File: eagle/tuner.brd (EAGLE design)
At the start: 42.8 x 53.3 mm, 32 parts, among them IC1 MEGA8-AI, IC2 LM358D, IC3 7805TV, M1 MIC

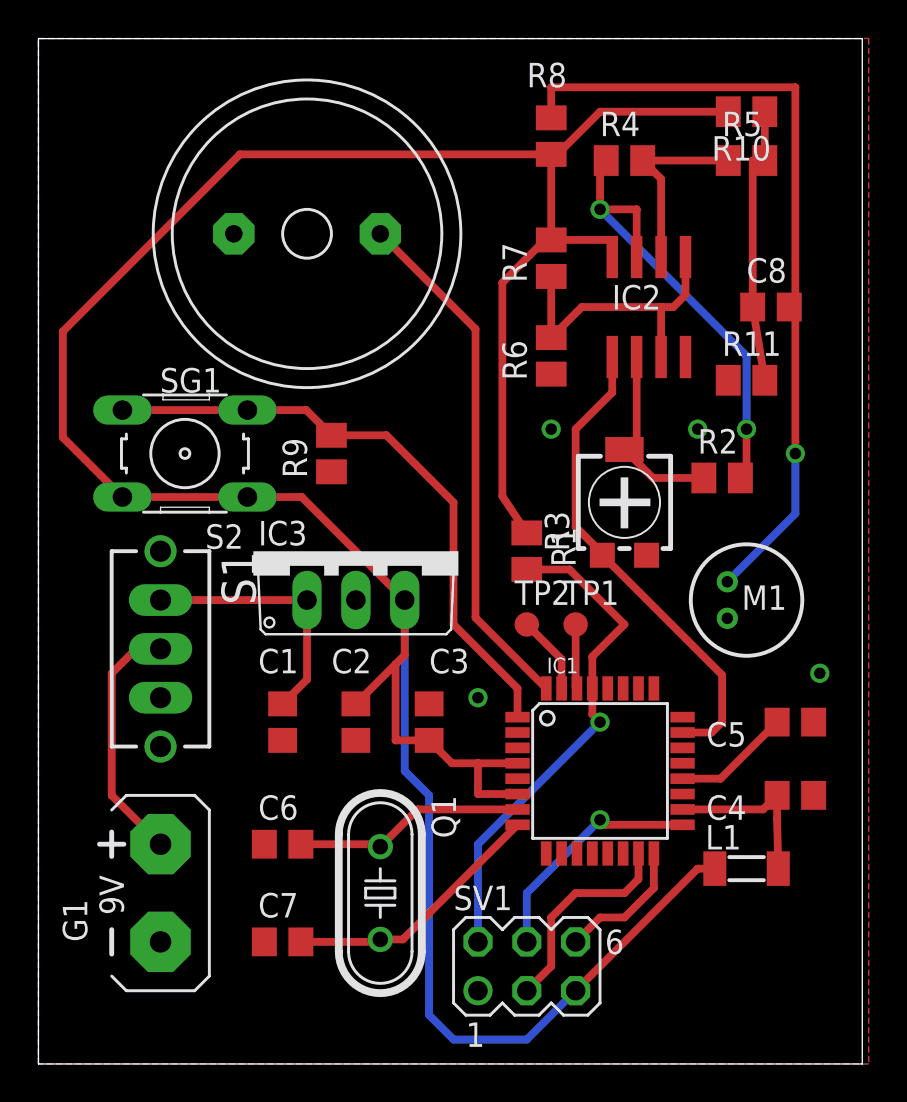
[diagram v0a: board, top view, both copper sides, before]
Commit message: updated PCB
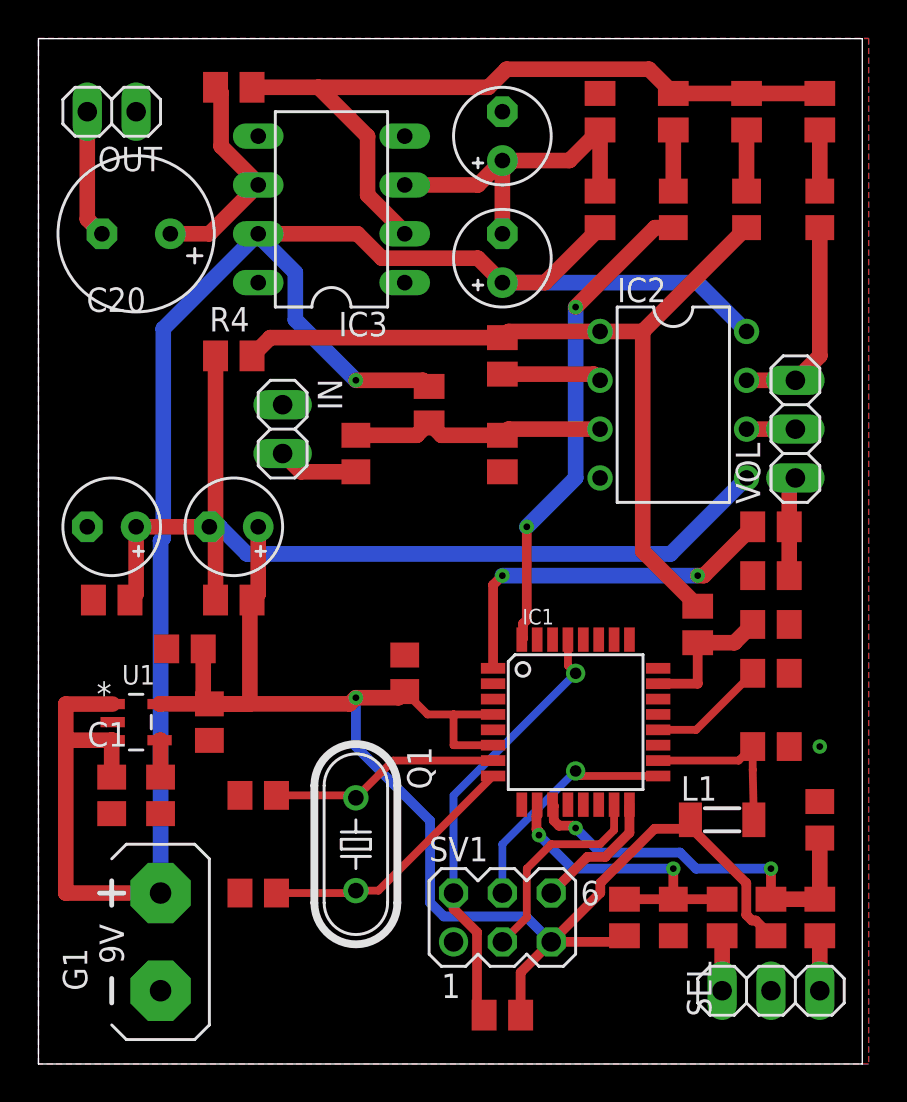
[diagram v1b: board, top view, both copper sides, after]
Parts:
- removed M1: MIC, microphon:WM-64PN
- removed S1: POWER, switch:TL3XYO
- removed S2: (no value), switch-omron:B3F-10XX
- removed SG1: BUZZER, buzzer:F/QMB
- removed TP1, TP2: PTR1B1,27, testpad:B1,27
- added C10, C14, C15, C22, C23: 0.1uF, eagle-ltspice:C0805
- added C11, C12, C13: 1uF, eagle-ltspice:C0805
- added C16, C17, C18, C19: 47uF, rcl:E2,5-5
- added C20: 470uF, rcl:E3,5-8
- added C9: 470pF, eagle-ltspice:C0805
- added IN, OUT: (no value), pinhead:1X02
- added R12, R13, R16, R17, R18, R19: 10k, resistor:M0805
- added R14, R15: 1k, resistor:M0805
- added SEL, VOL: (no value), pinhead:1X03
- added U1: LP2985AIM5-5.0, LP2985AIM5-5.0:SOT95P284X119-5N
- C2: value 0.1uF -> 2.2uF
- IC2: value LM358D -> LM358N; device linear:SO08 -> linear:DIL08
- IC3: value 7805TV -> AD811N; device linear:TO220V -> analog-devices:DIL08
- R10, R4: value 220k -> 10k
- R11: value 220k -> 20k
- R2: value 2.2k -> 100k
- R3: value (none) -> 100k; device resistor:RTRIM4G/J -> resistor:M0805
- R5, R8: value 2.2k -> 10k
- moved C8 35.3 mm to (30.5, 48.3)
- moved R6 26.2 mm to (26.7, 50.8), turned to 0 degrees
- moved R9 25.1 mm to (55.9, 76.2)
- moved R7 24.3 mm to (33.0, 50.8), turned to 0 degrees
- moved R1 24.2 mm to (47.0, 29.2), turned to 180 degrees
- moved R4 22.7 mm to (33.0, 63.5)
- moved IC3 17.8 mm to (38.1, 71.1), turned to 90 degrees
- moved R8 16.7 mm to (33.0, 77.5), turned to 180 degrees
- moved R5 16.3 mm to (47.0, 63.5), turned to 270 degrees
- moved R11 14.0 mm to (59.7, 76.2), turned to 90 degrees
- moved R2 11.5 mm to (47.0, 58.4), turned to 90 degrees
- moved R3 11.4 mm to (43.2, 61.0), turned to 90 degrees
- moved C1 9.67 mm to (26.7, 40.6)
- moved C2 7.62 mm to (31.8, 44.5)
- moved IC2 5.24 mm to (55.9, 61.0), turned to 270 degrees
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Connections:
- removed net RX: IC1.30, TP1.TP
- removed net TX: IC1.31, TP2.TP
- removed net V/2: IC2.3, IC2.5, R6.2, R7.1
- removed net VCC: C2.1, C3.2, IC1.4, IC1.6, IC2.8, IC3.3, L1.1, R1.1, R10.2, R7.2, R8.2, S2.1, S2.2, SV1.5
- new net 2.5V: C18.-, C19.+, IC2.5, R4.1, R6.2, R7.1
- new net 4.5V: C16.-, C17.+, IC3.3, R12.2, R13.1
- new net 5V: C18.+, C2.1, C3.2, C8.2, IC1.4, IC1.6, L1.1, R1.1, R18.2, R19.2, R7.2, SV1.5, U1.5
- new net 9V: C1.1, C16.+, G1.+, IC2.8, IC3.7, R13.2, R3.2, U1.1, U1.3
- new net CLICK: C10.1, IC1.32
- new net COUNT: C23.2, IC1.11, R17.2, R19.1
- new net INSTR: C12.1, IC2.1, R14.2, R4.2, R5.1
- new net N$11: IC3.2, R10.2, R11.2, R8.1, R9.2
- new net N$19: C15.1, R15.2, VOL.1
- new net N$20: IC2.6, VOL.2
- new net N$21: C20.-, OUT.2
- new net N$23: R16.1, SEL.1
- new net N$24: R17.1, SEL.3
- new net PHASE: C22.1, IC1.10, R16.2, R18.1
- new net TUNE: C11.1, IC2.7, VOL.3
- net GND: now also C14.1, C15.2, C17.-, C19.-, C22.2, C23.1, C8.1, C9.2, IC3.4, IN.1, OUT.1, R12.1, R2.1, SEL.2, U1.2; no longer IC3.2, M1.2, R11.1, R9.1, SG1.+
- net N$10: now also C13.1, IC2.3, R2.2; no longer IC1.23, IC2.1
- net N$12: now also C13.2, IN.2; no longer IC2.7, R2.2, R4.1
- net N$13: now also IC2.2, R5.2; no longer IC2.6, R4.2, R5.1
- net N$14: now also C10.2, R9.1; no longer C8.2, M1.1, R8.1
- net N$15: now also C14.2, IC1.23, R14.1; no longer C8.1, R10.1, R11.2, R5.2
- net N$16: now also C11.2, R10.1; no longer G1.+, S1.2
- net N$17: now also C12.2, R11.1; no longer IC1.1, R9.2, S2.3, S2.4
- net N$18: now also IC1.1, R15.1; no longer IC2.2, R2.1, R3.2
- net N$2: now also C9.1, U1.4; no longer C1.1, IC3.1, S1.1
- net N$9: now also C20.+, IC3.6, R8.2; no longer IC1.32, SG1.-
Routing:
- net VCC: track 154.2 -> 0.00 mm
- net 9V: track 0.00 -> 105.4 mm, vias 0 -> 1
- net 5V: track 0.00 -> 82.0 mm, vias 0 -> 1
- net 2.5V: track 0.00 -> 50.9 mm
- net INSTR: track 0.00 -> 44.0 mm
- net N$11: track 0.00 -> 39.9 mm
- net N$14: track 41.9 -> 3.18 mm, vias 1 -> 0
- net N$17: track 31.8 -> 3.18 mm
- net CLICK: track 0.00 -> 25.2 mm, vias 0 -> 2
- net COUNT: track 0.00 -> 20.5 mm, vias 0 -> 2
- net N$12: track 24.3 -> 4.20 mm, vias 2 -> 0
- net 4.5V: track 0.00 -> 18.5 mm
- net PHASE: track 0.00 -> 16.0 mm, vias 0 -> 2
- net V/2: track 15.7 -> 0.00 mm
- net N$9: track 27.2 -> 11.6 mm
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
